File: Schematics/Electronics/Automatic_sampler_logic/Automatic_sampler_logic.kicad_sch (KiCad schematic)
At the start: 14 parts, among them J1 MOT_X_SOCK_2, J2 MOT_X_SOCK_1, J3 MOT_Y_SOCK, J4 Power, J5 FINAL_SOCK, J6 MOT_Z_SOCK, U4 Pico, U5 LM7805_TO220

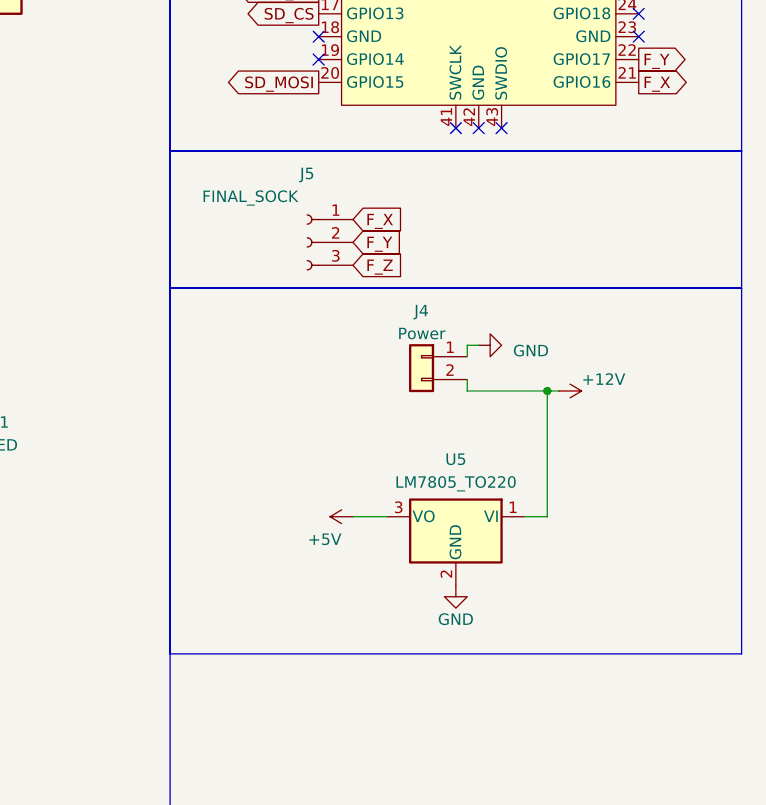
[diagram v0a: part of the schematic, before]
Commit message: Updating schematic
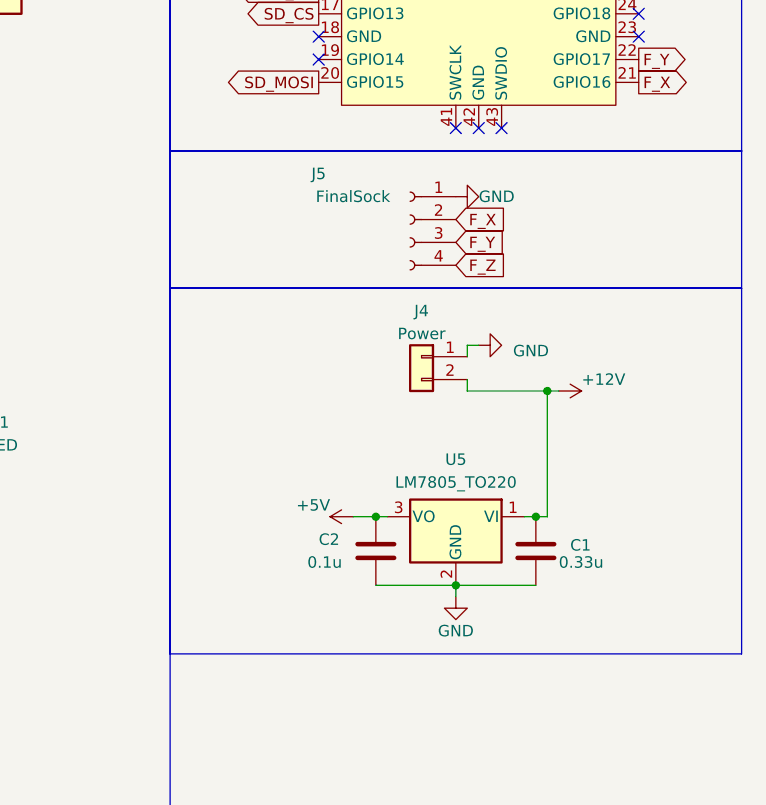
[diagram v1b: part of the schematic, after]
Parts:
- removed J5: FINAL_SOCK, Connector_PinSocket_2.54mm:PinSocket_1x03_P2.54mm_Vertical, symbol Connector:Conn_01x03_Socket
- added C1: 0.33u, symbol Device:C
- added C2: 0.1u, symbol Device:C
- added J5: FinalSock, Connector_PinSocket_2.54mm:PinSocket_1x04_P2.54mm_Vertical, symbol Connector:Conn_01x04_Socket
- D1: footprint (none) -> LED_THT:LED_D5.0mm
- J1, J2, J3, J6: footprint (none) -> Connector_JST:JST_PH_B4B-PH-K_1x04_P2.00mm_Vertical
- R1: footprint (none) -> Resistor_THT:R_Axial_DIN0207_L6.3mm_D2.5mm_P7.62mm_Horizontal
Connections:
- net +12V: now also C1.1
- net +5V: now also C2.1
- net F_X: now also J5.2 (Pin_2)
- net F_Y: now also J5.3 (Pin_3)
- net F_Z: now also J5.4 (Pin_4)
- net GND: now also C1.2, C2.2, J5.1 (Pin_1)

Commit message: Update Automatic_sampler_logic.kicad_sch
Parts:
- C2: footprint (none) -> Capacitor_THT:C_Disc_D6.0mm_W2.5mm_P5.00mm
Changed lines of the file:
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@@
       (effects (font (size 1.27 1.27)) (justify left))
     )
-    (property "Footprint" "" (at 141.9352 125.73 0)
+    (property "Footprint" "Capacitor_THT:C_Disc_D6.0mm_W2.5mm_P5.00mm" (at 141.9352 125.73 0)
       (effects (font (size 1.27 1.27)) hide)
     )

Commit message: Made PCB for AS
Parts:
- C1: footprint (none) -> Capacitor_THT:C_Disc_D6.0mm_W2.5mm_P5.00mm
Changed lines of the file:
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@@
       (effects (font (size 1.27 1.27)) (justify left))
     )
-    (property "Footprint" "" (at 159.7152 125.73 0)
+    (property "Footprint" "Capacitor_THT:C_Disc_D6.0mm_W2.5mm_P5.00mm" (at 159.7152 125.73 0)
       (effects (font (size 1.27 1.27)) hide)
     )
